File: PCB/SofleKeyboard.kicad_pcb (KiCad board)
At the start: 2 copper layers, 137.2 x 109.2 mm, 87 parts, among them J1 LED, J2 4PIN, J3 OLED, P1 i2c_pin, P2 i2c_pin, SW1 SW_PUSH, SW10 SW_PUSH, SW11 SW_PUSH, SW12 SW_PUSH, SW13 SW_PUSH, SW14 SW_PUSH, SW15 SW_PUSH, SW16 SW_PUSH, SW17 SW_PUSH, SW18 SW_PUSH, SW19 SW_PUSH, SW2 SW_PUSH, SW20 SW_PUSH, SW21 SW_PUSH, SW22 SW_PUSH, SW23 SW_PUSH, SW24 SW_PUSH, SW25 Rotary_Encoder_Switch, SW26 SW_PUSH, SW27 SW_PUSH, SW28 SW_PUSH, SW29 SW_PUSH, SW3 SW_PUSH, SW30 SW_PUSH, SW4 SW_PUSH, SW5 SW_PUSH, SW6 SW_PUSH, SW7 SW_PUSH, SW8 SW_PUSH, SW9 SW_PUSH, U1 ProMicro

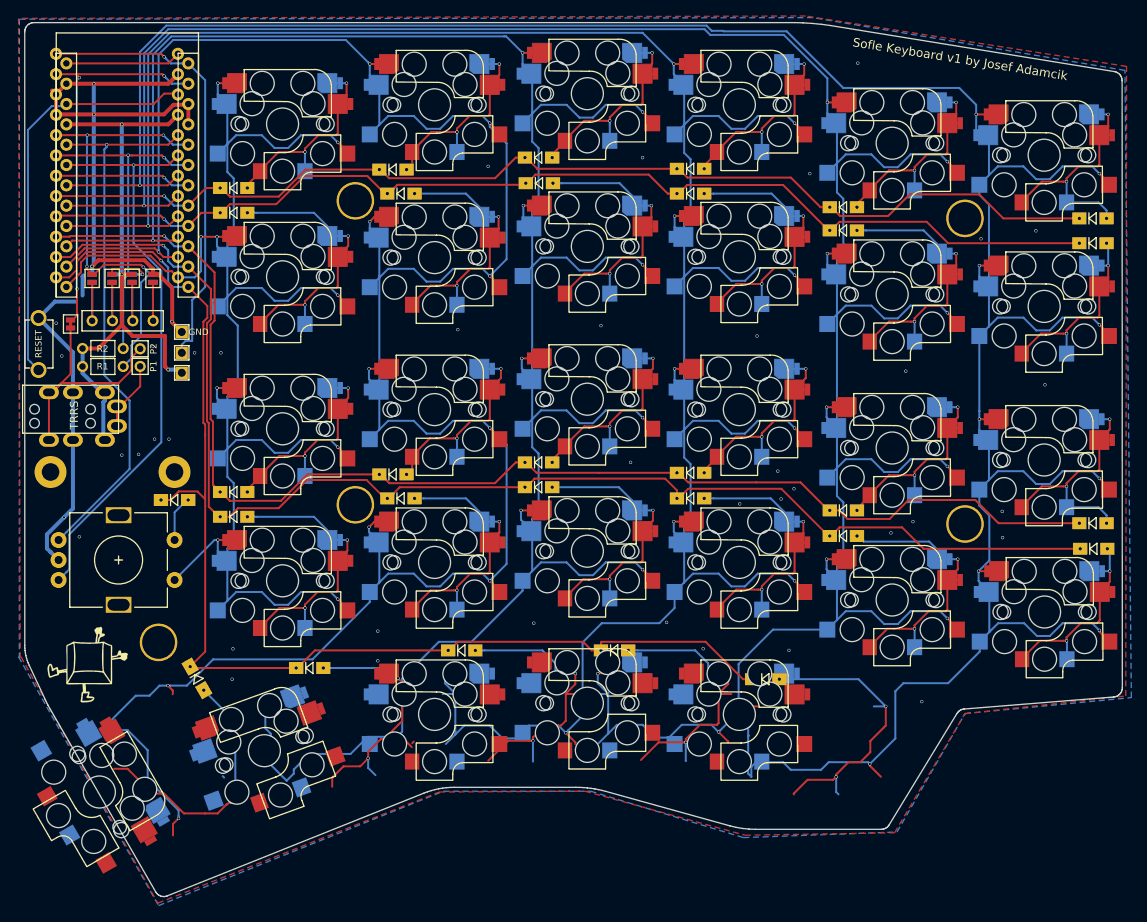
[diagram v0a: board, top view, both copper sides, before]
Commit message: WIP changing the stagger
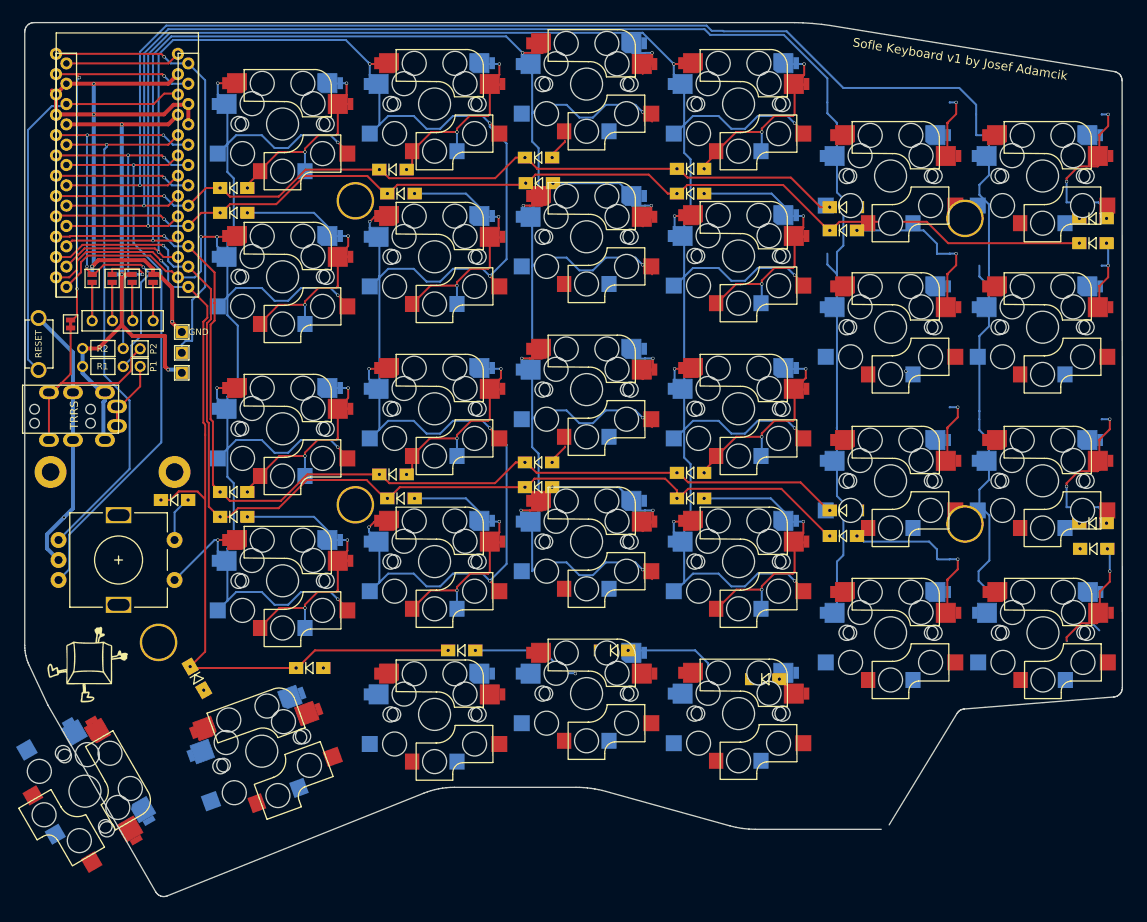
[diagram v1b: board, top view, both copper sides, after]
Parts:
- moved SW11 4.10 mm to (196.5, 75.4)
- moved SW5 4.10 mm to (196.5, 56.5)
- moved SW17 4.10 mm to (196.5, 94.6)
- moved SW23 4.10 mm to (196.5, 113.6)
- moved SW12 2.61 mm to (215.5, 75.4)
- moved SW6 2.61 mm to (215.5, 56.5)
- moved SW18 2.61 mm to (215.5, 94.6)
- moved SW24 2.61 mm to (215.6, 113.6)
- moved SW26 1.80 mm to (95.8, 133.4)
- moved SW15 1.20 mm to (158.5, 83.2)
- moved SW21 1.20 mm to (158.5, 102.2)
- moved SW29 1.20 mm to (158.5, 121.2)
- moved SW3 1.20 mm to (158.5, 45.0)
- moved SW9 1.20 mm to (158.5, 64.1)
- moved SW27 0.33 mm to (117.9, 128.4)
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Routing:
- net col1: track 350.6 -> 195.4 mm, vias 11 -> 1
- net col0: track 354.5 -> 213.9 mm, vias 10 -> 1
- net col3: track 314.7 -> 242.6 mm, vias 11 -> 9
- net col4: track 311.0 -> 250.5 mm, vias 11 -> 9
- net col2: track 334.4 -> 275.1 mm, vias 11 -> 9
- net row4: track 152.5 -> 110.7 mm
- net Net-(D30-Pad2): track 37.0 -> 0.00 mm, vias 2 -> 0
- net Net-(D26-Pad2): track 36.4 -> 0.00 mm, vias 2 -> 0
- net row2: track 165.8 -> 131.9 mm
- net row0: track 138.2 -> 104.3 mm
- net Net-(D27-Pad2): track 32.8 -> 0.00 mm, vias 2 -> 0
- net row3: track 170.1 -> 137.4 mm
- net Net-(D28-Pad2): track 37.1 -> 14.5 mm, vias 2 -> 1
- net Net-(D29-Pad2): track 36.9 -> 14.5 mm, vias 2 -> 0
- net Net-(D5-Pad2): track 27.9 -> 7.92 mm, vias 2 -> 1
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- removed copper zone on B.Cu, net GND
- removed copper zone on F.Cu, net GND
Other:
- outline, holes or cut-outs redrawn
